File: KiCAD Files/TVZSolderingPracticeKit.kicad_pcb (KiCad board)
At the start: 2 copper layers, 100 x 100 mm, 51 parts, among them J1 Barrel Jack, J2 Conn_01x05_Pin, J3 Conn_01x05_Socket, J4 Conn_01x03_Pin, J5 Conn_01x03_Pin, SW1 SW_Push, SW10 POWER, SW11 C/D, SW2 SW_Push, SW3 SW_Push, SW4 SW_Push, SW5 SW_Push, SW6 SW_Push, SW7 SW_Push, SW8 SW_Push, U1 NE555P

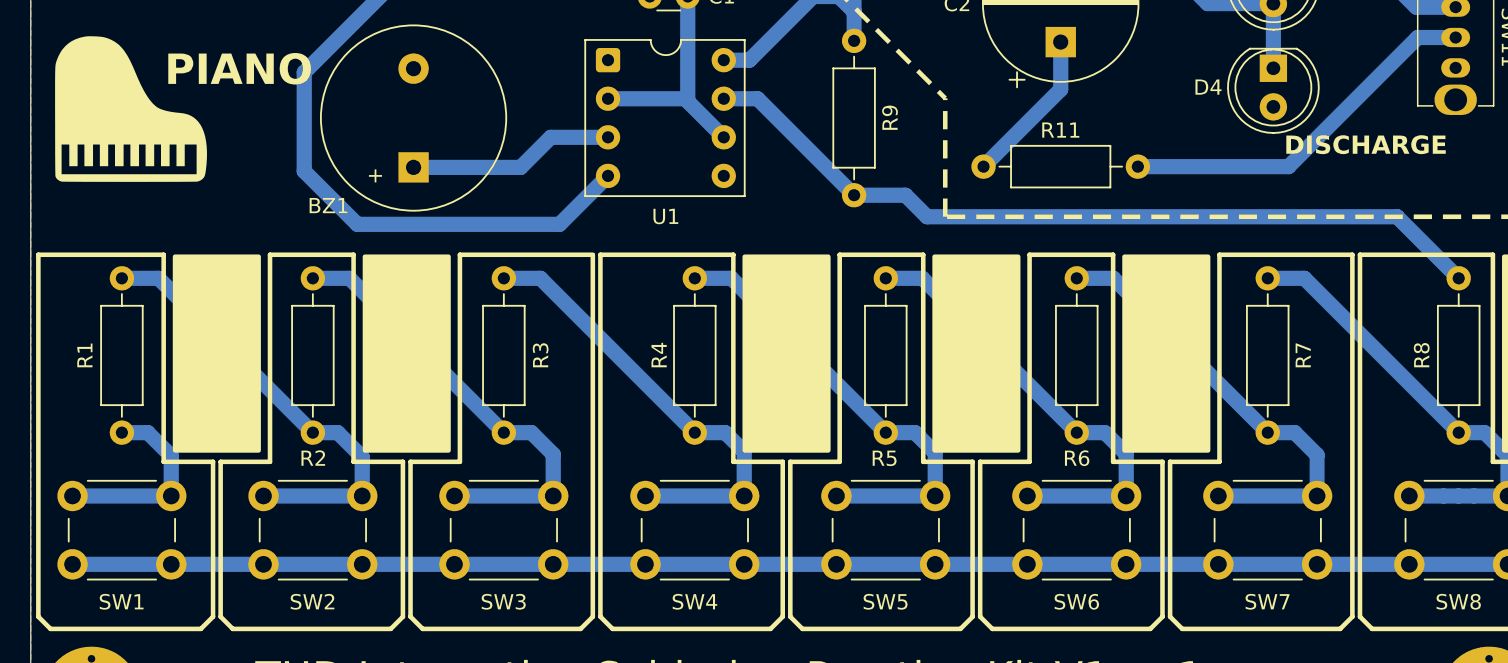
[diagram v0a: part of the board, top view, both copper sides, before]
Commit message: update
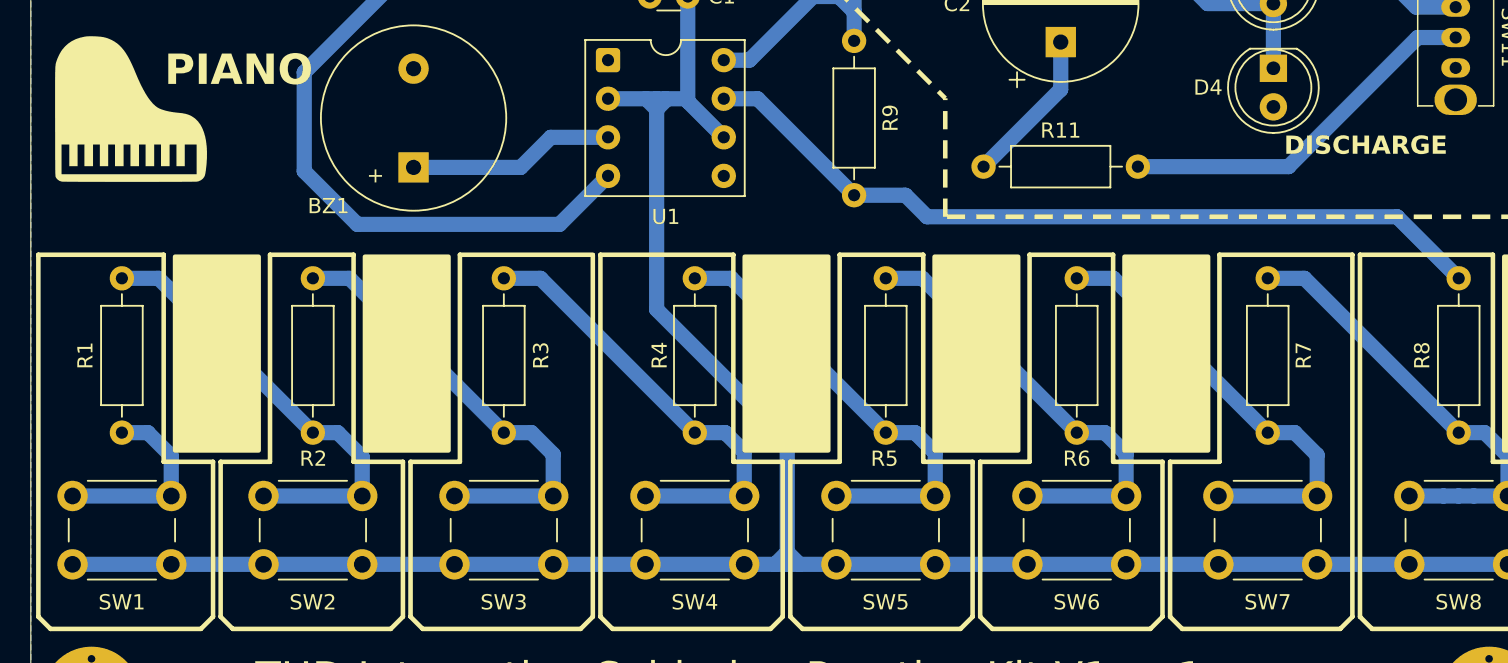
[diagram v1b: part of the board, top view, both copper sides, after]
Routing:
- net Net-(U1-THR): track 110.1 -> 148.5 mm
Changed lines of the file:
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@@
 			)
 		)
-		(property "Datasheet" ""
+		(property "Datasheet" "~"
 			(at 0 0 180)
 			(unlocked yes)
@@
 			)
 		)
-		(property "Datasheet" ""
+		(property "Datasheet" "~"
 			(at 0 0 180)
 			(unlocked yes)
@@
 			)
 		)
-		(property "Datasheet" ""
+		(property "Datasheet" "~"
 			(at 0 0 90)
 			(layer "F.Fab")
@@
 			)
 		)
-		(property "Datasheet" ""
+		(property "Datasheet" "~"
 			(at 0 0 90)
 			(unlocked yes)
@@
 			)
 		)
-		(property "Datasheet" ""
+		(property "Datasheet" "~"
 			(at 0 0 270)
 			(unlocked yes)
@@
 			)
 		)
-		(property "Datasheet" ""
+		(property "Datasheet" "~"
 			(at 0 0 90)
 			(unlocked yes)
@@
 			)
 		)
-		(property "Datasheet" ""
+		(property "Datasheet" "~"
 			(at 0 0 0)
 			(layer "F.Fab")
@@
 			)
 		)
-		(property "Datasheet" ""
+		(property "Datasheet" "~"
 			(at 0 0 270)
 			(unlocked yes)
@@
 			)
 		)
-		(property "Datasheet" ""
+		(property "Datasheet" "~"
 			(at 0 0 180)
 			(unlocked yes)
@@
 			)
 		)
-		(property "Datasheet" ""
+		(property "Datasheet" "~"
 			(at 0 0 90)
 			(unlocked yes)
@@
 			)
 		)
-		(property "Datasheet" ""
+		(property "Datasheet" "~"
 			(at 0 0 270)
 			(unlocked yes)
@@
 			)
 		)
-		(property "Datasheet" ""
+		(property "Datasheet" "~"
 			(at 0 0 0)
 			(unlocked yes)
@@
 			)
 		)
-		(property "Datasheet" ""
+		(property "Datasheet" "~"
 			(at 0 0 270)
 			(unlocked yes)
@@
 			)
 		)
-		(property "Datasheet" ""
+		(property "Datasheet" "~"
 			(at 0 0 0)
 			(unlocked yes)
@@
 			)
 		)
-		(property "Datasheet" ""
+		(property "Datasheet" "~"
 			(at 0 0 270)
 			(unlocked yes)
@@
 			)
 		)
-		(property "Datasheet" ""
+		(property "Datasheet" "~"
 			(at 0 0 270)
 			(unlocked yes)
@@
 			)
 		)
-		(property "Datasheet" ""
+		(property "Datasheet" "~"
 			(at 0 0 180)
 			(unlocked yes)
@@
 			)
 		)
-		(property "Datasheet" ""
+		(property "Datasheet" "~"
 			(at 0 0 90)
 			(unlocked yes)
@@
 			)
 		)
-		(property "Datasheet" ""
+		(property "Datasheet" "~"
 			(at 0 0 270)
 			(unlocked yes)
@@
 			)
 		)
-		(property "Datasheet" ""
+		(property "Datasheet" "~"
 			(at 0 0 0)
 			(unlocked yes)
@@
 			)
 		)
-		(property "Datasheet" ""
+		(property "Datasheet" "~"
 			(at 0 0 90)
 			(layer "F.Fab")
@@
 			)
 		)
-		(property "Datasheet" ""
+		(property "Datasheet" "~"
 			(at 0 0 0)
 			(unlocked yes)
@@
 			)
 		)
-		(property "Datasheet" ""
+		(property "Datasheet" "~"
 			(at 0 0 270)
 			(unlocked yes)
@@
 			)
 		)
-		(property "Datasheet" ""
+		(property "Datasheet" "~"
 			(at 0 0 90)
 			(layer "F.Fab")
@@
 			)
 		)
-		(property "Datasheet" ""
+		(property "Datasheet" "~"
 			(at 0 0 270)
 			(unlocked yes)
@@
 			)
 		)
-		(property "Datasheet" ""
+		(property "Datasheet" "~"
 			(at 0 0 0)
 			(unlocked yes)
@@
 			)
 		)
-		(property "Datasheet" ""
+		(property "Datasheet" "~"
 			(at 0 0 270)
 			(unlocked yes)
@@
 			)
 		)
-		(property "Datasheet" ""
+		(property "Datasheet" "~"
 			(at 0 0 90)
 			(layer "F.Fab")
@@
 			)
 		)
-		(property "Datasheet" ""
+		(property "Datasheet" "~"
 			(at 0 0 0)
 			(layer "F.Fab")
@@
 			)
 		)
-		(property "Datasheet" ""
+		(property "Datasheet" "~"
 			(at 0 0 90)
 			(layer "F.Fab")
@@
 			)
 		)
-		(property "Datasheet" ""
+		(property "Datasheet" "~"
 			(at 0 0 90)
 			(unlocked yes)
@@
 			)
 		)
-		(property "Datasheet" ""
+		(property "Datasheet" "~"
 			(at 0 0 90)
 			(layer "F.Fab")
@@
 			)
 		)
-		(property "Datasheet" ""
+		(property "Datasheet" "~"
 			(at 0 0 0)
 			(unlocked yes)
@@
 			)
 		)
-		(property "Datasheet" ""
+		(property "Datasheet" "~"
 			(at 0 0 270)
 			(unlocked yes)
@@
 			)
 		)
-		(property "Datasheet" ""
+		(property "Datasheet" "~"
 			(at 0 0 0)
 			(layer "F.Fab")
@@
 			)
 		)
-		(property "Datasheet" ""
+		(property "Datasheet" "~"
 			(at 0 0 90)
 			(layer "F.Fab")
@@
 			)
 		)
-		(property "Datasheet" ""
+		(property "Datasheet" "~"
 			(at 0 0 0)
 			(unlocked yes)
@@
 			)
 		)
-		(property "Datasheet" ""
+		(property "Datasheet" "~"
 			(at 0 0 0)
 			(layer "F.Fab")
@@
 			)
 		)
-		(property "Datasheet" ""
+		(property "Datasheet" "~"
 			(at 0 0 90)
 			(layer "F.Fab")
@@
 			)
 		)
-		(property "Datasheet" ""
+		(property "Datasheet" "~"
 			(at 0 0 270)
 			(unlocked yes)
@@
 			)
 		)
-		(property "Datasheet" ""
+		(property "Datasheet" "~"
 			(at 0 0 90)
 			(unlocked yes)
@@
 			)
 		)
-		(property "Datasheet" ""
+		(property "Datasheet" "~"
 			(at 0 0 0)
 			(unlocked yes)
@@
 			)
 		)
-		(property "Datasheet" ""
+		(property "Datasheet" "~"
 			(at 0 0 0)
 			(layer "F.Fab")
@@
 			)
 		)
-		(property "Datasheet" ""
+		(property "Datasheet" "~"
 			(at 0 0 0)
 			(unlocked yes)
@@
 			)
 		)
-		(property "Datasheet" ""
+		(property "Datasheet" "~"
 			(at 0 0 0)
 			(layer "F.Fab")
@@
 	)
 	(segment
+		(start 99.78 167.1)
+		(end 99 167.88)
+		(width 1)
+		(layer "B.Cu")
+		(net 1)
+	)
+	(segment
+		(start 91.8 137.33)
+		(end 91.8 137.23)
+		(width 1)
+		(layer "B.Cu")
+		(net 1)
+	)
+	(segment
 		(start 147.25 167.88)
 		(end 140.75 167.88)
@@
 	)
 	(segment
+		(start 99.8 167.1)
+		(end 99.82 167.1)
+		(width 1)
+		(layer "B.Cu")
+		(net 1)
+	)
+	(segment
+		(start 99.8 167.1)
+		(end 99.8 159.7)
+		(width 1)
+		(layer "B.Cu")
+		(net 1)
+	)
+	(segment
 		(start 88 137.23)
-		(end 93.08 137.23)
+		(end 90.5 137.23)
 		(width 1)
 		(layer "B.Cu")
@@
 	)
 	(segment
+		(start 91.2 138)
+		(end 91.2 137.93)
+		(width 1)
+		(layer "B.Cu")
+		(net 1)
+	)
+	(segment
 		(start 93.25 137.4)
 		(end 95.62 139.77)
@@
 	)
 	(segment
+		(start 91.2 137.93)
+		(end 90.5 137.23)
+		(width 1)
+		(layer "B.Cu")
+		(net 1)
+	)
+	(segment
+		(start 90.5 137.23)
+		(end 91.2 137.23)
+		(width 1)
+		(layer "B.Cu")
+		(net 1)
+	)
+	(segment
+		(start 99.82 167.1)
+		(end 100.6 167.88)
+		(width 1)
+		(layer "B.Cu")
+		(net 1)
+	)
+	(segment
+		(start 91.2 137.23)
+		(end 91.8 137.23)
+		(width 1)
+		(layer "B.Cu")
+		(net 1)
+	)
+	(segment
+		(start 91.2 137.23)
+		(end 91.2 138)
+		(width 1)
+		(layer "B.Cu")
+		(net 1)
+	)
+	(segment
+		(start 91.8 137.23)
+		(end 93.08 137.23)
+		(width 1)
+		(layer "B.Cu")
+		(net 1)
+	)
+	(segment
+		(start 99.8 167.88)
+		(end 99.8 167.1)
+		(width 1)
+		(layer "B.Cu")
+		(net 1)
+	)
+	(segment
+		(start 100.6 167.88)
+		(end 99.8 167.88)
+		(width 1)
+		(layer "B.Cu")
+		(net 1)
+	)
+	(segment
+		(start 91.2 138)
+		(end 91.2 151.1)
+		(width 1)
+		(layer "B.Cu")
+		(net 1)
+	)
+	(segment
 		(start 93.25 130.5)
 		(end 93.25 137.4)
@@
 	)
 	(segment
-		(start 140.75 167.88)
+		(start 99.8 159.7)
+		(end 91.2 151.1)
+		(width 1)
+		(layer "B.Cu")
+		(net 1)
+	)
+	(segment
+		(start 99.8 167.88)
+		(end 99 167.88)
+		(width 1)
+		(layer "B.Cu")
+		(net 1)
+	)
+	(segment
+		(start 99 167.88)
 		(end 52.75 167.88)
 		(width 1)
 		(layer "B.Cu")
+		(net 1)
+	)
+	(segment
+		(start 91.2 137.93)
+		(end 91.8 137.33)
+		(width 1)
+		(layer "B.Cu")
+		(net 1)
+	)
+	(segment
+		(start 140.75 167.88)
+		(end 100.6 167.88)
+		(width 1)
+		(layer "B.Cu")
+		(net 1)
+	)
+	(segment
+		(start 99.8 167.1)
+		(end 99.78 167.1)
+		(width 1)
+		(layer "B.Cu")
